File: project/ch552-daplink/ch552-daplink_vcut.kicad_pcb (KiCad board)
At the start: 2 copper layers, 92 x 92 mm, 512 parts, among them J1 USB_C_Receptacle_USB2.0_16P, J10 USB_C_Receptacle_USB2.0_16P, J11 Conn_01x06_Pin, J12 BOOT, J13 USB_C_Receptacle_USB2.0_16P, J14 Conn_01x06_Pin, J15 BOOT, J16 USB_C_Receptacle_USB2.0_16P, J17 Conn_01x06_Pin, J18 BOOT, J19 USB_C_Receptacle_USB2.0_16P, J2 Conn_01x06_Pin, J20 Conn_01x06_Pin, J21 BOOT, J22 USB_C_Receptacle_USB2.0_16P, J23 Conn_01x06_Pin, J24 BOOT, J25 USB_C_Receptacle_USB2.0_16P, J26 Conn_01x06_Pin, J27 BOOT, J28 USB_C_Receptacle_USB2.0_16P, J29 Conn_01x06_Pin, J3 BOOT, J30 BOOT, J31 USB_C_Receptacle_USB2.0_16P, J32 Conn_01x06_Pin, J33 BOOT, J34 USB_C_Receptacle_USB2.0_16P, J35 Conn_01x06_Pin, J36 BOOT, J37 USB_C_Receptacle_USB2.0_16P, J38 Conn_01x06_Pin, J39 BOOT, J4 USB_C_Receptacle_USB2.0_16P, J40 USB_C_Receptacle_USB2.0_16P, J41 Conn_01x06_Pin, J42 BOOT, J43 USB_C_Receptacle_USB2.0_16P, J44 Conn_01x06_Pin, J45 BOOT, J46 USB_C_Receptacle_USB2.0_16P, J47 Conn_01x06_Pin, J48 BOOT, J49 USB_C_Receptacle_USB2.0_16P, J5 Conn_01x06_Pin, J50 Conn_01x06_Pin, J51 BOOT, J52 USB_C_Receptacle_USB2.0_16P, J53 Conn_01x06_Pin, J54 BOOT, J55 USB_C_Receptacle_USB2.0_16P, J56 Conn_01x06_Pin, J57 BOOT, J58 USB_C_Receptacle_USB2.0_16P, J59 Conn_01x06_Pin, J6 BOOT, J60 BOOT, J61 USB_C_Receptacle_USB2.0_16P, J62 Conn_01x06_Pin, J63 BOOT, J64 USB_C_Receptacle_USB2.0_16P, J65 Conn_01x06_Pin, J66 BOOT, J67 USB_C_Receptacle_USB2.0_16P, J68 Conn_01x06_Pin, J69 BOOT, J7 USB_C_Receptacle_USB2.0_16P, J70 USB_C_Receptacle_USB2.0_16P, J71 Conn_01x06_Pin, J72 BOOT, J73 USB_C_Receptacle_USB2.0_16P, J74 Conn_01x06_Pin, J75 BOOT, J76 USB_C_Receptacle_USB2.0_16P, J77 Conn_01x06_Pin, J78 BOOT, J79 USB_C_Receptacle_USB2.0_16P, J8 Conn_01x06_Pin, J80 Conn_01x06_Pin, J81 BOOT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

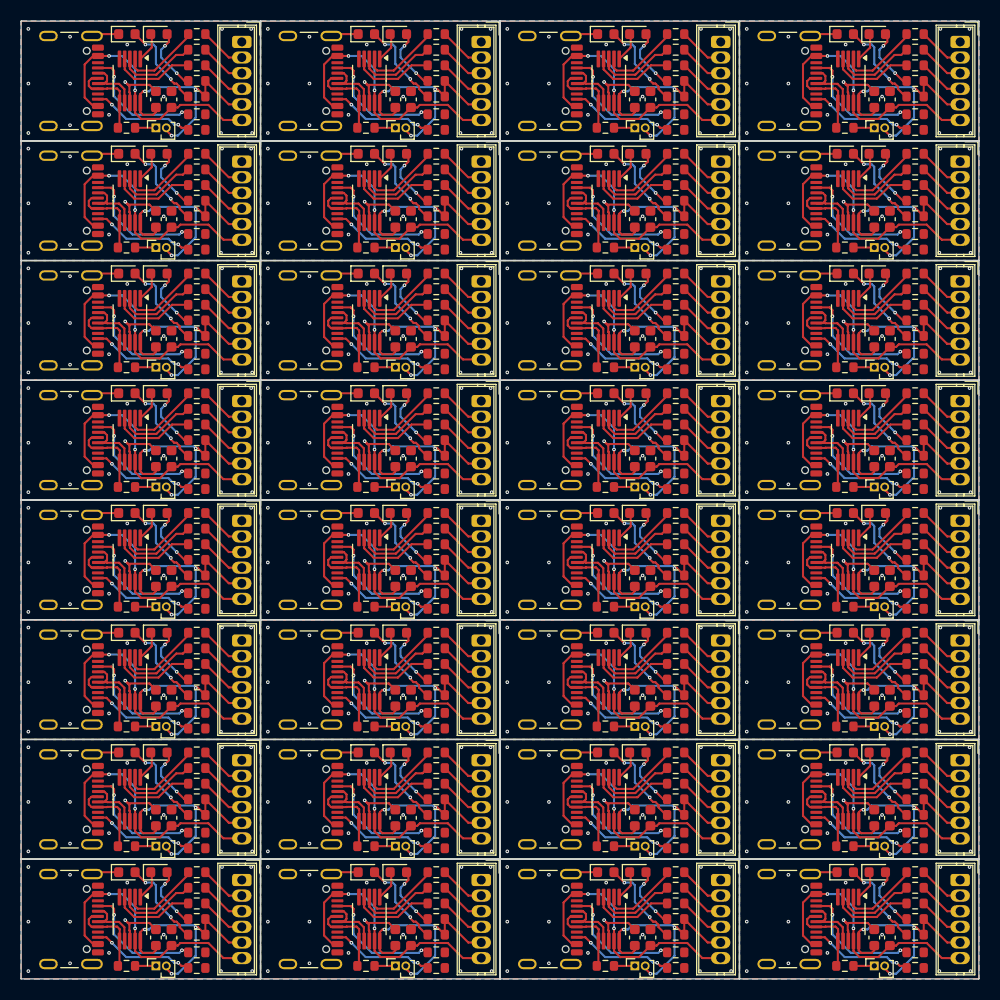
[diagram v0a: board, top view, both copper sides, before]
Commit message: 2025/07/20/17:06
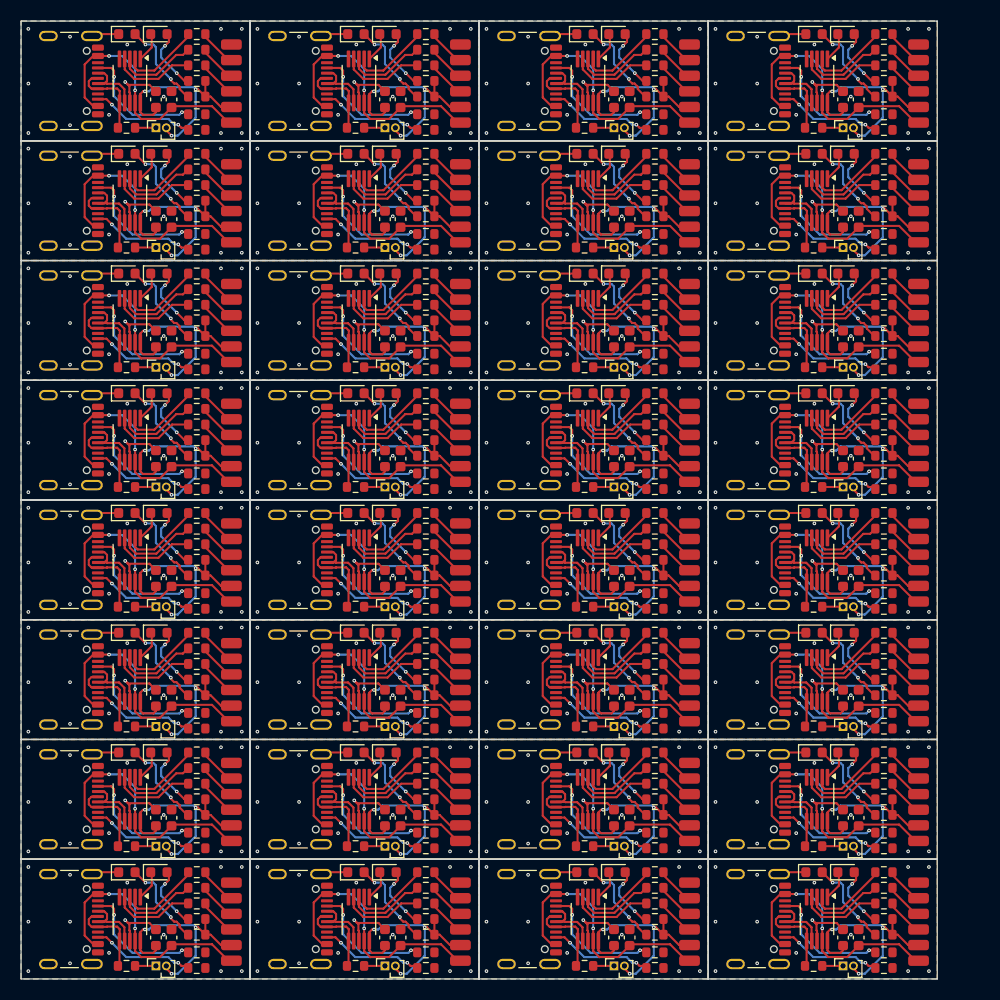
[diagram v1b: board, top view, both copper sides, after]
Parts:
- removed the C1 at (139.4, 175.5)
- removed C10, C11, C12, C13, C14, C15, C16, C17, C18, C19, C20, C21, C22, C23, C24, C25, C26, C27, C28, C29, C3, C30, C31, C32, C33, C34, C35, C36, C37, C38, C39, C4, C40, C41, C42, C43, C44, C45, C46, C47, C48, C49, C5, C50, C51, C52, C53, C54, C55, C56, C57, C58, C59, C6, C60, C61, C62, C63, C64, C7, C8, C9: 0.1uF, Capacitor_SMD:C_0603_1608Metric
- removed the C2 at (140.9, 175.5)
- removed the D1 at (136.7, 169.2)
- removed D10, D12, D14, D16, D18, D20, D22, D24, D26, D28, D30, D32, D34, D36, D38, D4, D40, D42, D44, D46, D48, D50, D52, D54, D56, D58, D6, D60, D62, D64, D8: Green, LED_SMD:LED_0603_1608Metric
- removed D11, D13, D15, D17, D19, D21, D23, D25, D27, D29, D3, D31, D33, D35, D37, D39, D41, D43, D45, D47, D49, D5, D51, D53, D55, D57, D59, D61, D63, D7, D9: Blue, LED_SMD:LED_0603_1608Metric
- removed the D2 at (139.7, 169.2)
- removed the J1 at (130.2, 173.8)
- removed J10, J13, J16, J19, J22, J25, J28, J31, J34, J37, J4, J40, J43, J46, J49, J52, J55, J58, J61, J64, J67, J7, J70, J73, J76, J79, J82, J85, J88, J91, J94: USB_C_Receptacle_USB2.0_16P, Connector_USB:USB_C_Receptacle_GCT_USB4105-xx-A_16P_TopMnt_Horizontal
- removed J11, J14, J17, J2, J20, J23, J26, J29, J32, J35, J38, J41, J44, J47, J5, J50, J53, J56, J59, J62, J65, J68, J71, J74, J77, J8, J80, J83, J86, J89, J92, J95: Conn_01x06_Pin, Connector_Wuerth:Wuerth_WR-WTB_64800611622_1x06_P1.50mm_Vertical
- removed J12, J15, J18, J21, J24, J27, J30, J33, J36, J39, J42, J45, J48, J51, J54, J57, J6, J60, J63, J66, J69, J72, J75, J78, J81, J84, J87, J9, J90, J93, J96: BOOT, Connector_PinSocket_1.00mm:PinSocket_1x02_P1.00mm_Vertical
- removed the J3 at (139.4, 178.2)
- removed the R1 at (143.4, 176.9)
- removed R10, R105, R106, R113, R114, R121, R122, R129, R130, R137, R138, R145, R146, R153, R154, R161, R162, R169, R17, R170, R177, R178, R18, R185, R186, R193, R194, R201, R202, R209, R210, R217, R218, R225, R226, R233, R234, R241, R242, R249, R25, R250, R26, R33, R34, R41, R42, R49, R50, R57, R58, R65, R66, R73, R74, R81, R82, R89, R9, R90, R97, R98: 5.1kΩ, Resistor_SMD:R_0603_1608Metric
- removed R100, R107, R108, R11, R115, R116, R12, R123, R124, R131, R132, R139, R140, R147, R148, R155, R156, R163, R164, R171, R172, R179, R180, R187, R188, R19, R195, R196, R20, R203, R204, R211, R212, R219, R220, R227, R228, R235, R236, R243, R244, R251, R252, R27, R28, R35, R36, R43, R44, R51, R52, R59, R60, R67, R68, R75, R76, R83, R84, R91, R92, R99: 1kΩ, Resistor_SMD:R_0603_1608Metric
- removed R101, R109, R117, R125, R13, R133, R141, R149, R157, R165, R173, R181, R189, R197, R205, R21, R213, R221, R229, R237, R245, R253, R29, R37, R45, R53, R61, R69, R77, R85, R93: 10kΩ, Resistor_SMD:R_0603_1608Metric
- removed R102, R103, R104, R110, R111, R112, R118, R119, R120, R126, R127, R128, R134, R135, R136, R14, R142, R143, R144, R15, R150, R151, R152, R158, R159, R16, R160, R166, R167, R168, R174, R175, R176, R182, R183, R184, R190, R191, R192, R198, R199, R200, R206, R207, R208, R214, R215, R216, R22, R222, R223, R224, R23, R230, R231, R232, R238, R239, R24, R240, R246, R247, R248, R254, R255, R256, R30, R31, R32, R38, R39, R40, R46, R47, R48, R54, R55, R56, R62, R63, R64, R70, R71, R72, R78, R79, R80, R86, R87, R88, R94, R95, R96: 100Ω, Resistor_SMD:R_0603_1608Metric
- removed the R2 at (143.4, 178.4)
- removed the R3 at (143.4, 175.2)
- removed the R4 at (143.4, 173.8)
- removed the R5 at (136.6, 178.2)
- removed the R6 at (143.4, 172.2)
- removed the R7 at (143.4, 170.8)
- removed the R8 at (143.4, 169.2)
- removed the U1 at (136.9, 173.8)
- removed U10, U11, U12, U13, U14, U15, U16, U17, U18, U19, U2, U20, U21, U22, U23, U24, U25, U26, U27, U28, U29, U3, U30, U31, U32, U4, U5, U6, U7, U8, U9: CH552E, Package_SO:MSOP-10_3x3mm_P0.5mm
- added C1: 0.1uF, Capacitor_SMD:C_0603_1608Metric, F.Cu at (92.5, 95.0)
- added C1: 0.1uF, Capacitor_SMD:C_0603_1608Metric, F.Cu at (92.5, 106.5)
- added C1: 0.1uF, Capacitor_SMD:C_0603_1608Metric, F.Cu at (70.5, 164.0)
- added C1: 0.1uF, Capacitor_SMD:C_0603_1608Metric, F.Cu at (70.5, 106.5)
- added C1: 0.1uF, Capacitor_SMD:C_0603_1608Metric, F.Cu at (136.4, 175.5)
- added C1: 0.1uF, Capacitor_SMD:C_0603_1608Metric, F.Cu at (92.5, 164.0)
- added C1: 0.1uF, Capacitor_SMD:C_0603_1608Metric, F.Cu at (70.5, 118.0)
- added C1: 0.1uF, Capacitor_SMD:C_0603_1608Metric, F.Cu at (70.5, 152.5)
- added C1: 0.1uF, Capacitor_SMD:C_0603_1608Metric, F.Cu at (92.5, 118.0)
- added C1: 0.1uF, Capacitor_SMD:C_0603_1608Metric, F.Cu at (114.5, 129.5)
- added C1: 0.1uF, Capacitor_SMD:C_0603_1608Metric, F.Cu at (136.4, 164.0)
- added C1: 0.1uF, Capacitor_SMD:C_0603_1608Metric, F.Cu at (114.5, 152.5)
- added C1: 0.1uF, Capacitor_SMD:C_0603_1608Metric, F.Cu at (70.5, 129.5)
- added C1: 0.1uF, Capacitor_SMD:C_0603_1608Metric, F.Cu at (114.5, 118.0)
- added C1: 0.1uF, Capacitor_SMD:C_0603_1608Metric, F.Cu at (136.4, 95.0)
- added C1: 0.1uF, Capacitor_SMD:C_0603_1608Metric, F.Cu at (70.5, 141.0)
- added C1: 0.1uF, Capacitor_SMD:C_0603_1608Metric, F.Cu at (136.4, 152.5)
- added C1: 0.1uF, Capacitor_SMD:C_0603_1608Metric, F.Cu at (114.5, 95.0)
- added C1: 0.1uF, Capacitor_SMD:C_0603_1608Metric, F.Cu at (92.5, 129.5)
- added C1: 0.1uF, Capacitor_SMD:C_0603_1608Metric, F.Cu at (136.4, 129.5)
- added C1: 0.1uF, Capacitor_SMD:C_0603_1608Metric, F.Cu at (92.5, 141.0)
- added C1: 0.1uF, Capacitor_SMD:C_0603_1608Metric, F.Cu at (70.5, 175.5)
- added C1: 0.1uF, Capacitor_SMD:C_0603_1608Metric, F.Cu at (92.5, 175.5)
- added C1: 0.1uF, Capacitor_SMD:C_0603_1608Metric, F.Cu at (92.5, 152.5)
- added C1: 0.1uF, Capacitor_SMD:C_0603_1608Metric, F.Cu at (136.4, 106.5)
- added C1: 0.1uF, Capacitor_SMD:C_0603_1608Metric, F.Cu at (114.5, 106.5)
- added C1: 0.1uF, Capacitor_SMD:C_0603_1608Metric, F.Cu at (70.5, 95.0)
- added C1: 0.1uF, Capacitor_SMD:C_0603_1608Metric, F.Cu at (136.4, 118.0)
- added C1: 0.1uF, Capacitor_SMD:C_0603_1608Metric, F.Cu at (114.5, 164.0)
- added C1: 0.1uF, Capacitor_SMD:C_0603_1608Metric, F.Cu at (114.5, 141.0)
- added C1: 0.1uF, Capacitor_SMD:C_0603_1608Metric, F.Cu at (114.5, 175.5)
- added C1: 0.1uF, Capacitor_SMD:C_0603_1608Metric, F.Cu at (136.4, 141.0)
- added C2: 0.1uF, Capacitor_SMD:C_0603_1608Metric, F.Cu at (116.0, 152.5)
- added C2: 0.1uF, Capacitor_SMD:C_0603_1608Metric, F.Cu at (94.0, 118.0)
- added C2: 0.1uF, Capacitor_SMD:C_0603_1608Metric, F.Cu at (116.0, 141.0)
- added C2: 0.1uF, Capacitor_SMD:C_0603_1608Metric, F.Cu at (94.0, 106.5)
- added C2: 0.1uF, Capacitor_SMD:C_0603_1608Metric, F.Cu at (137.9, 152.5)
- added C2: 0.1uF, Capacitor_SMD:C_0603_1608Metric, F.Cu at (72.0, 129.5)
- added C2: 0.1uF, Capacitor_SMD:C_0603_1608Metric, F.Cu at (72.0, 95.0)
- added C2: 0.1uF, Capacitor_SMD:C_0603_1608Metric, F.Cu at (137.9, 95.0)
- added C2: 0.1uF, Capacitor_SMD:C_0603_1608Metric, F.Cu at (116.0, 164.0)
- added C2: 0.1uF, Capacitor_SMD:C_0603_1608Metric, F.Cu at (72.0, 175.5)
- added C2: 0.1uF, Capacitor_SMD:C_0603_1608Metric, F.Cu at (116.0, 129.5)
- added C2: 0.1uF, Capacitor_SMD:C_0603_1608Metric, F.Cu at (116.0, 95.0)
- added C2: 0.1uF, Capacitor_SMD:C_0603_1608Metric, F.Cu at (116.0, 106.5)
- added C2: 0.1uF, Capacitor_SMD:C_0603_1608Metric, F.Cu at (94.0, 175.5)
- added C2: 0.1uF, Capacitor_SMD:C_0603_1608Metric, F.Cu at (94.0, 129.5)
- added C2: 0.1uF, Capacitor_SMD:C_0603_1608Metric, F.Cu at (94.0, 95.0)
- added C2: 0.1uF, Capacitor_SMD:C_0603_1608Metric, F.Cu at (72.0, 118.0)
- added C2: 0.1uF, Capacitor_SMD:C_0603_1608Metric, F.Cu at (137.9, 141.0)
- added C2: 0.1uF, Capacitor_SMD:C_0603_1608Metric, F.Cu at (137.9, 106.5)
- added C2: 0.1uF, Capacitor_SMD:C_0603_1608Metric, F.Cu at (116.0, 118.0)
- added C2: 0.1uF, Capacitor_SMD:C_0603_1608Metric, F.Cu at (72.0, 164.0)
- added C2: 0.1uF, Capacitor_SMD:C_0603_1608Metric, F.Cu at (94.0, 164.0)
- added C2: 0.1uF, Capacitor_SMD:C_0603_1608Metric, F.Cu at (137.9, 118.0)
- added C2: 0.1uF, Capacitor_SMD:C_0603_1608Metric, F.Cu at (94.0, 152.5)
- added C2: 0.1uF, Capacitor_SMD:C_0603_1608Metric, F.Cu at (72.0, 141.0)
- added C2: 0.1uF, Capacitor_SMD:C_0603_1608Metric, F.Cu at (137.9, 164.0)
- added C2: 0.1uF, Capacitor_SMD:C_0603_1608Metric, F.Cu at (72.0, 106.5)
- added C2: 0.1uF, Capacitor_SMD:C_0603_1608Metric, F.Cu at (72.0, 152.5)
- added C2: 0.1uF, Capacitor_SMD:C_0603_1608Metric, F.Cu at (116.0, 175.5)
- added C2: 0.1uF, Capacitor_SMD:C_0603_1608Metric, F.Cu at (137.9, 129.5)
- added C2: 0.1uF, Capacitor_SMD:C_0603_1608Metric, F.Cu at (94.0, 141.0)
- added C2: 0.1uF, Capacitor_SMD:C_0603_1608Metric, F.Cu at (137.9, 175.5)
- added D1: Blue, LED_SMD:LED_0603_1608Metric, F.Cu at (133.7, 146.2)
- added D1: Blue, LED_SMD:LED_0603_1608Metric, F.Cu at (133.7, 123.2)
- added D1: Blue, LED_SMD:LED_0603_1608Metric, F.Cu at (89.7, 100.2)
- added D1: Blue, LED_SMD:LED_0603_1608Metric, F.Cu at (133.7, 88.8)
- added D1: Blue, LED_SMD:LED_0603_1608Metric, F.Cu at (67.7, 146.2)
- added D1: Blue, LED_SMD:LED_0603_1608Metric, F.Cu at (133.7, 169.2)
- added D1: Blue, LED_SMD:LED_0603_1608Metric, F.Cu at (133.7, 111.8)
- added D1: Blue, LED_SMD:LED_0603_1608Metric, F.Cu at (89.7, 123.2)
- added D1: Blue, LED_SMD:LED_0603_1608Metric, F.Cu at (133.7, 100.2)
- added D1: Blue, LED_SMD:LED_0603_1608Metric, F.Cu at (67.7, 123.2)
- added D1: Blue, LED_SMD:LED_0603_1608Metric, F.Cu at (111.7, 169.2)
- added D1: Blue, LED_SMD:LED_0603_1608Metric, F.Cu at (67.7, 100.2)
- added D1: Blue, LED_SMD:LED_0603_1608Metric, F.Cu at (67.7, 88.8)
- added D1: Blue, LED_SMD:LED_0603_1608Metric, F.Cu at (89.7, 88.8)
- added D1: Blue, LED_SMD:LED_0603_1608Metric, F.Cu at (89.7, 146.2)
- added D1: Blue, LED_SMD:LED_0603_1608Metric, F.Cu at (111.7, 100.2)
- added D1: Blue, LED_SMD:LED_0603_1608Metric, F.Cu at (111.7, 123.2)
- added D1: Blue, LED_SMD:LED_0603_1608Metric, F.Cu at (111.7, 111.8)
- added D1: Blue, LED_SMD:LED_0603_1608Metric, F.Cu at (111.7, 88.8)
- added D1: Blue, LED_SMD:LED_0603_1608Metric, F.Cu at (89.7, 134.8)
- added D1: Blue, LED_SMD:LED_0603_1608Metric, F.Cu at (133.7, 134.8)
- added D1: Blue, LED_SMD:LED_0603_1608Metric, F.Cu at (67.7, 111.8)
- added D1: Blue, LED_SMD:LED_0603_1608Metric, F.Cu at (89.7, 111.8)
- added D1: Blue, LED_SMD:LED_0603_1608Metric, F.Cu at (89.7, 169.2)
- added D1: Blue, LED_SMD:LED_0603_1608Metric, F.Cu at (111.7, 157.8)
- added D1: Blue, LED_SMD:LED_0603_1608Metric, F.Cu at (67.7, 134.8)
- added D1: Blue, LED_SMD:LED_0603_1608Metric, F.Cu at (133.7, 157.8)
- added D1: Blue, LED_SMD:LED_0603_1608Metric, F.Cu at (67.7, 169.2)
- added D1: Blue, LED_SMD:LED_0603_1608Metric, F.Cu at (89.7, 157.8)
- added D1: Blue, LED_SMD:LED_0603_1608Metric, F.Cu at (67.7, 157.8)
- added D1: Blue, LED_SMD:LED_0603_1608Metric, F.Cu at (111.7, 134.8)
- added D1: Blue, LED_SMD:LED_0603_1608Metric, F.Cu at (111.7, 146.2)
- added D2: Green, LED_SMD:LED_0603_1608Metric, F.Cu at (92.7, 100.2)
- added D2: Green, LED_SMD:LED_0603_1608Metric, F.Cu at (136.7, 134.8)
- added D2: Green, LED_SMD:LED_0603_1608Metric, F.Cu at (136.7, 157.8)
- added D2: Green, LED_SMD:LED_0603_1608Metric, F.Cu at (92.7, 146.2)
- added D2: Green, LED_SMD:LED_0603_1608Metric, F.Cu at (114.7, 111.8)
- added D2: Green, LED_SMD:LED_0603_1608Metric, F.Cu at (70.7, 88.8)
- added D2: Green, LED_SMD:LED_0603_1608Metric, F.Cu at (70.7, 157.8)
- added D2: Green, LED_SMD:LED_0603_1608Metric, F.Cu at (114.7, 134.8)
- added D2: Green, LED_SMD:LED_0603_1608Metric, F.Cu at (136.7, 88.8)
- added D2: Green, LED_SMD:LED_0603_1608Metric, F.Cu at (92.7, 157.8)
- added D2: Green, LED_SMD:LED_0603_1608Metric, F.Cu at (70.7, 123.2)
- added D2: Green, LED_SMD:LED_0603_1608Metric, F.Cu at (70.7, 111.8)
- added D2: Green, LED_SMD:LED_0603_1608Metric, F.Cu at (114.7, 88.8)
- added D2: Green, LED_SMD:LED_0603_1608Metric, F.Cu at (92.7, 134.8)
- added D2: Green, LED_SMD:LED_0603_1608Metric, F.Cu at (70.7, 169.2)
- added D2: Green, LED_SMD:LED_0603_1608Metric, F.Cu at (136.7, 146.2)
- added D2: Green, LED_SMD:LED_0603_1608Metric, F.Cu at (92.7, 123.2)
- added D2: Green, LED_SMD:LED_0603_1608Metric, F.Cu at (136.7, 169.2)
- added D2: Green, LED_SMD:LED_0603_1608Metric, F.Cu at (136.7, 123.2)
- added D2: Green, LED_SMD:LED_0603_1608Metric, F.Cu at (114.7, 123.2)
- added D2: Green, LED_SMD:LED_0603_1608Metric, F.Cu at (70.7, 134.8)
- added D2: Green, LED_SMD:LED_0603_1608Metric, F.Cu at (114.7, 169.2)
- added D2: Green, LED_SMD:LED_0603_1608Metric, F.Cu at (114.7, 146.2)
- added D2: Green, LED_SMD:LED_0603_1608Metric, F.Cu at (92.7, 88.8)
- added D2: Green, LED_SMD:LED_0603_1608Metric, F.Cu at (136.7, 100.2)
- added D2: Green, LED_SMD:LED_0603_1608Metric, F.Cu at (70.7, 100.2)
- added D2: Green, LED_SMD:LED_0603_1608Metric, F.Cu at (70.7, 146.2)
- added D2: Green, LED_SMD:LED_0603_1608Metric, F.Cu at (92.7, 169.2)
- added D2: Green, LED_SMD:LED_0603_1608Metric, F.Cu at (92.7, 111.8)
- added D2: Green, LED_SMD:LED_0603_1608Metric, F.Cu at (114.7, 157.8)
- added D2: Green, LED_SMD:LED_0603_1608Metric, F.Cu at (136.7, 111.8)
- added D2: Green, LED_SMD:LED_0603_1608Metric, F.Cu at (114.7, 100.2)
- added J1: USB_C_Receptacle_USB2.0_16P, Connector_USB:USB_C_Receptacle_GCT_USB4105-xx-A_16P_TopMnt_Horizontal, F.Cu at (61.2, 104.8)
- added J1: USB_C_Receptacle_USB2.0_16P, Connector_USB:USB_C_Receptacle_GCT_USB4105-xx-A_16P_TopMnt_Horizontal, F.Cu at (83.2, 93.2)
- added J1: USB_C_Receptacle_USB2.0_16P, Connector_USB:USB_C_Receptacle_GCT_USB4105-xx-A_16P_TopMnt_Horizontal, F.Cu at (127.2, 93.2)
- added J1: USB_C_Receptacle_USB2.0_16P, Connector_USB:USB_C_Receptacle_GCT_USB4105-xx-A_16P_TopMnt_Horizontal, F.Cu at (61.2, 162.2)
- added J1: USB_C_Receptacle_USB2.0_16P, Connector_USB:USB_C_Receptacle_GCT_USB4105-xx-A_16P_TopMnt_Horizontal, F.Cu at (105.2, 150.8)
- added J1: USB_C_Receptacle_USB2.0_16P, Connector_USB:USB_C_Receptacle_GCT_USB4105-xx-A_16P_TopMnt_Horizontal, F.Cu at (127.2, 150.8)
- added J1: USB_C_Receptacle_USB2.0_16P, Connector_USB:USB_C_Receptacle_GCT_USB4105-xx-A_16P_TopMnt_Horizontal, F.Cu at (105.2, 104.8)
- added J1: USB_C_Receptacle_USB2.0_16P, Connector_USB:USB_C_Receptacle_GCT_USB4105-xx-A_16P_TopMnt_Horizontal, F.Cu at (127.2, 139.2)
- added J1: USB_C_Receptacle_USB2.0_16P, Connector_USB:USB_C_Receptacle_GCT_USB4105-xx-A_16P_TopMnt_Horizontal, F.Cu at (127.2, 173.8)
- added J1: USB_C_Receptacle_USB2.0_16P, Connector_USB:USB_C_Receptacle_GCT_USB4105-xx-A_16P_TopMnt_Horizontal, F.Cu at (61.2, 127.8)
- added J1: USB_C_Receptacle_USB2.0_16P, Connector_USB:USB_C_Receptacle_GCT_USB4105-xx-A_16P_TopMnt_Horizontal, F.Cu at (61.2, 116.2)
- added J1: USB_C_Receptacle_USB2.0_16P, Connector_USB:USB_C_Receptacle_GCT_USB4105-xx-A_16P_TopMnt_Horizontal, F.Cu at (61.2, 139.2)
- added J1: USB_C_Receptacle_USB2.0_16P, Connector_USB:USB_C_Receptacle_GCT_USB4105-xx-A_16P_TopMnt_Horizontal, F.Cu at (105.2, 127.8)
- added J1: USB_C_Receptacle_USB2.0_16P, Connector_USB:USB_C_Receptacle_GCT_USB4105-xx-A_16P_TopMnt_Horizontal, F.Cu at (105.2, 173.8)
- added J1: USB_C_Receptacle_USB2.0_16P, Connector_USB:USB_C_Receptacle_GCT_USB4105-xx-A_16P_TopMnt_Horizontal, F.Cu at (105.2, 139.2)
- added J1: USB_C_Receptacle_USB2.0_16P, Connector_USB:USB_C_Receptacle_GCT_USB4105-xx-A_16P_TopMnt_Horizontal, F.Cu at (83.2, 127.8)
- added J1: USB_C_Receptacle_USB2.0_16P, Connector_USB:USB_C_Receptacle_GCT_USB4105-xx-A_16P_TopMnt_Horizontal, F.Cu at (105.2, 116.2)
- added J1: USB_C_Receptacle_USB2.0_16P, Connector_USB:USB_C_Receptacle_GCT_USB4105-xx-A_16P_TopMnt_Horizontal, F.Cu at (83.2, 116.2)
- added J1: USB_C_Receptacle_USB2.0_16P, Connector_USB:USB_C_Receptacle_GCT_USB4105-xx-A_16P_TopMnt_Horizontal, F.Cu at (61.2, 93.2)
- added J1: USB_C_Receptacle_USB2.0_16P, Connector_USB:USB_C_Receptacle_GCT_USB4105-xx-A_16P_TopMnt_Horizontal, F.Cu at (83.2, 139.2)
- added J1: USB_C_Receptacle_USB2.0_16P, Connector_USB:USB_C_Receptacle_GCT_USB4105-xx-A_16P_TopMnt_Horizontal, F.Cu at (83.2, 162.2)
- added J1: USB_C_Receptacle_USB2.0_16P, Connector_USB:USB_C_Receptacle_GCT_USB4105-xx-A_16P_TopMnt_Horizontal, F.Cu at (83.2, 150.8)
- added J1: USB_C_Receptacle_USB2.0_16P, Connector_USB:USB_C_Receptacle_GCT_USB4105-xx-A_16P_TopMnt_Horizontal, F.Cu at (127.2, 116.2)
- added J1: USB_C_Receptacle_USB2.0_16P, Connector_USB:USB_C_Receptacle_GCT_USB4105-xx-A_16P_TopMnt_Horizontal, F.Cu at (127.2, 104.8)
- added J1: USB_C_Receptacle_USB2.0_16P, Connector_USB:USB_C_Receptacle_GCT_USB4105-xx-A_16P_TopMnt_Horizontal, F.Cu at (105.2, 162.2)
- added J1: USB_C_Receptacle_USB2.0_16P, Connector_USB:USB_C_Receptacle_GCT_USB4105-xx-A_16P_TopMnt_Horizontal, F.Cu at (105.2, 93.2)
- added J1: USB_C_Receptacle_USB2.0_16P, Connector_USB:USB_C_Receptacle_GCT_USB4105-xx-A_16P_TopMnt_Horizontal, F.Cu at (127.2, 127.8)
- added J1: USB_C_Receptacle_USB2.0_16P, Connector_USB:USB_C_Receptacle_GCT_USB4105-xx-A_16P_TopMnt_Horizontal, F.Cu at (83.2, 173.8)
- added J1: USB_C_Receptacle_USB2.0_16P, Connector_USB:USB_C_Receptacle_GCT_USB4105-xx-A_16P_TopMnt_Horizontal, F.Cu at (61.2, 173.8)
- added J1: USB_C_Receptacle_USB2.0_16P, Connector_USB:USB_C_Receptacle_GCT_USB4105-xx-A_16P_TopMnt_Horizontal, F.Cu at (127.2, 162.2)
- added J1: USB_C_Receptacle_USB2.0_16P, Connector_USB:USB_C_Receptacle_GCT_USB4105-xx-A_16P_TopMnt_Horizontal, F.Cu at (61.2, 150.8)
- added J1: USB_C_Receptacle_USB2.0_16P, Connector_USB:USB_C_Receptacle_GCT_USB4105-xx-A_16P_TopMnt_Horizontal, F.Cu at (83.2, 104.8)
- added J3: BOOT, Connector_PinSocket_1.00mm:PinSocket_1x02_P1.00mm_Vertical, F.Cu at (70.5, 132.2)
- added J3: BOOT, Connector_PinSocket_1.00mm:PinSocket_1x02_P1.00mm_Vertical, F.Cu at (92.5, 155.2)
- added J3: BOOT, Connector_PinSocket_1.00mm:PinSocket_1x02_P1.00mm_Vertical, F.Cu at (70.5, 143.8)
- added J3: BOOT, Connector_PinSocket_1.00mm:PinSocket_1x02_P1.00mm_Vertical, F.Cu at (70.5, 97.8)
- added J3: BOOT, Connector_PinSocket_1.00mm:PinSocket_1x02_P1.00mm_Vertical, F.Cu at (114.5, 178.2)
- added J3: BOOT, Connector_PinSocket_1.00mm:PinSocket_1x02_P1.00mm_Vertical, F.Cu at (70.5, 120.8)
- added J3: BOOT, Connector_PinSocket_1.00mm:PinSocket_1x02_P1.00mm_Vertical, F.Cu at (136.4, 178.2)
- added J3: BOOT, Connector_PinSocket_1.00mm:PinSocket_1x02_P1.00mm_Vertical, F.Cu at (114.5, 97.8)
- added J3: BOOT, Connector_PinSocket_1.00mm:PinSocket_1x02_P1.00mm_Vertical, F.Cu at (92.5, 109.2)
- added J3: BOOT, Connector_PinSocket_1.00mm:PinSocket_1x02_P1.00mm_Vertical, F.Cu at (70.5, 166.8)
- added J3: BOOT, Connector_PinSocket_1.00mm:PinSocket_1x02_P1.00mm_Vertical, F.Cu at (70.5, 109.2)
- added J3: BOOT, Connector_PinSocket_1.00mm:PinSocket_1x02_P1.00mm_Vertical, F.Cu at (136.4, 166.8)
- added J3: BOOT, Connector_PinSocket_1.00mm:PinSocket_1x02_P1.00mm_Vertical, F.Cu at (70.5, 155.2)
- added J3: BOOT, Connector_PinSocket_1.00mm:PinSocket_1x02_P1.00mm_Vertical, F.Cu at (114.5, 143.8)
- added J3: BOOT, Connector_PinSocket_1.00mm:PinSocket_1x02_P1.00mm_Vertical, F.Cu at (136.4, 132.2)
- added J3: BOOT, Connector_PinSocket_1.00mm:PinSocket_1x02_P1.00mm_Vertical, F.Cu at (136.4, 97.8)
- added J3: BOOT, Connector_PinSocket_1.00mm:PinSocket_1x02_P1.00mm_Vertical, F.Cu at (114.5, 120.8)
- added J3: BOOT, Connector_PinSocket_1.00mm:PinSocket_1x02_P1.00mm_Vertical, F.Cu at (92.5, 97.8)
- added J3: BOOT, Connector_PinSocket_1.00mm:PinSocket_1x02_P1.00mm_Vertical, F.Cu at (92.5, 178.2)
- added J3: BOOT, Connector_PinSocket_1.00mm:PinSocket_1x02_P1.00mm_Vertical, F.Cu at (70.5, 178.2)
- added J3: BOOT, Connector_PinSocket_1.00mm:PinSocket_1x02_P1.00mm_Vertical, F.Cu at (92.5, 120.8)
- added J3: BOOT, Connector_PinSocket_1.00mm:PinSocket_1x02_P1.00mm_Vertical, F.Cu at (92.5, 132.2)
- added J3: BOOT, Connector_PinSocket_1.00mm:PinSocket_1x02_P1.00mm_Vertical, F.Cu at (136.4, 120.8)
- added J3: BOOT, Connector_PinSocket_1.00mm:PinSocket_1x02_P1.00mm_Vertical, F.Cu at (92.5, 143.8)
- added J3: BOOT, Connector_PinSocket_1.00mm:PinSocket_1x02_P1.00mm_Vertical, F.Cu at (136.4, 155.2)
- added J3: BOOT, Connector_PinSocket_1.00mm:PinSocket_1x02_P1.00mm_Vertical, F.Cu at (114.5, 132.2)
- added J3: BOOT, Connector_PinSocket_1.00mm:PinSocket_1x02_P1.00mm_Vertical, F.Cu at (136.4, 143.8)
- added J3: BOOT, Connector_PinSocket_1.00mm:PinSocket_1x02_P1.00mm_Vertical, F.Cu at (92.5, 166.8)
- added J3: BOOT, Connector_PinSocket_1.00mm:PinSocket_1x02_P1.00mm_Vertical, F.Cu at (114.5, 166.8)
- added J3: BOOT, Connector_PinSocket_1.00mm:PinSocket_1x02_P1.00mm_Vertical, F.Cu at (114.5, 109.2)
- added J3: BOOT, Connector_PinSocket_1.00mm:PinSocket_1x02_P1.00mm_Vertical, F.Cu at (114.5, 155.2)
- added J3: BOOT, Connector_PinSocket_1.00mm:PinSocket_1x02_P1.00mm_Vertical, F.Cu at (136.4, 109.2)
- added R1: 5.1kΩ, Resistor_SMD:R_0603_1608Metric, F.Cu at (140.4, 108.0)
- added R1: 5.1kΩ, Resistor_SMD:R_0603_1608Metric, F.Cu at (74.4, 153.9)
- added R1: 5.1kΩ, Resistor_SMD:R_0603_1608Metric, F.Cu at (96.4, 119.5)
- added R1: 5.1kΩ, Resistor_SMD:R_0603_1608Metric, F.Cu at (140.4, 130.9)
- added R1: 5.1kΩ, Resistor_SMD:R_0603_1608Metric, F.Cu at (140.4, 96.5)
- added R1: 5.1kΩ, Resistor_SMD:R_0603_1608Metric, F.Cu at (74.4, 96.5)
- added R1: 5.1kΩ, Resistor_SMD:R_0603_1608Metric, F.Cu at (118.4, 176.9)
- added R1: 5.1kΩ, Resistor_SMD:R_0603_1608Metric, F.Cu at (96.4, 153.9)
- added R1: 5.1kΩ, Resistor_SMD:R_0603_1608Metric, F.Cu at (140.4, 142.4)
- added R1: 5.1kΩ, Resistor_SMD:R_0603_1608Metric, F.Cu at (74.4, 176.9)
- added R1: 5.1kΩ, Resistor_SMD:R_0603_1608Metric, F.Cu at (118.4, 142.4)
- added R1: 5.1kΩ, Resistor_SMD:R_0603_1608Metric, F.Cu at (118.4, 108.0)
- added R1: 5.1kΩ, Resistor_SMD:R_0603_1608Metric, F.Cu at (74.4, 119.5)
- added R1: 5.1kΩ, Resistor_SMD:R_0603_1608Metric, F.Cu at (118.4, 153.9)
- added R1: 5.1kΩ, Resistor_SMD:R_0603_1608Metric, F.Cu at (74.4, 165.4)
- added R1: 5.1kΩ, Resistor_SMD:R_0603_1608Metric, F.Cu at (96.4, 108.0)
- added R1: 5.1kΩ, Resistor_SMD:R_0603_1608Metric, F.Cu at (96.4, 176.9)
- added R1: 5.1kΩ, Resistor_SMD:R_0603_1608Metric, F.Cu at (96.4, 142.4)
- added R1: 5.1kΩ, Resistor_SMD:R_0603_1608Metric, F.Cu at (118.4, 119.5)
- added R1: 5.1kΩ, Resistor_SMD:R_0603_1608Metric, F.Cu at (140.4, 165.4)
- added R1: 5.1kΩ, Resistor_SMD:R_0603_1608Metric, F.Cu at (74.4, 108.0)
- added R1: 5.1kΩ, Resistor_SMD:R_0603_1608Metric, F.Cu at (74.4, 130.9)
- added R1: 5.1kΩ, Resistor_SMD:R_0603_1608Metric, F.Cu at (140.4, 176.9)
- added R1: 5.1kΩ, Resistor_SMD:R_0603_1608Metric, F.Cu at (96.4, 96.5)
- added R1: 5.1kΩ, Resistor_SMD:R_0603_1608Metric, F.Cu at (118.4, 165.4)
- added R1: 5.1kΩ, Resistor_SMD:R_0603_1608Metric, F.Cu at (118.4, 96.5)
- added R1: 5.1kΩ, Resistor_SMD:R_0603_1608Metric, F.Cu at (96.4, 165.4)
- added R1: 5.1kΩ, Resistor_SMD:R_0603_1608Metric, F.Cu at (118.4, 130.9)
- added R1: 5.1kΩ, Resistor_SMD:R_0603_1608Metric, F.Cu at (140.4, 119.5)
- added R1: 5.1kΩ, Resistor_SMD:R_0603_1608Metric, F.Cu at (74.4, 142.4)
- added R1: 5.1kΩ, Resistor_SMD:R_0603_1608Metric, F.Cu at (96.4, 130.9)
- added R1: 5.1kΩ, Resistor_SMD:R_0603_1608Metric, F.Cu at (140.4, 153.9)
- added R2: 5.1kΩ, Resistor_SMD:R_0603_1608Metric, F.Cu at (118.4, 109.5)
- added R2: 5.1kΩ, Resistor_SMD:R_0603_1608Metric, F.Cu at (74.4, 109.5)
- added R2: 5.1kΩ, Resistor_SMD:R_0603_1608Metric, F.Cu at (96.4, 178.4)
- added R2: 5.1kΩ, Resistor_SMD:R_0603_1608Metric, F.Cu at (96.4, 121.0)
- added R2: 5.1kΩ, Resistor_SMD:R_0603_1608Metric, F.Cu at (74.4, 155.4)
- added R2: 5.1kΩ, Resistor_SMD:R_0603_1608Metric, F.Cu at (96.4, 109.5)
- added R2: 5.1kΩ, Resistor_SMD:R_0603_1608Metric, F.Cu at (118.4, 121.0)
- added R2: 5.1kΩ, Resistor_SMD:R_0603_1608Metric, F.Cu at (96.4, 166.9)
- added R2: 5.1kΩ, Resistor_SMD:R_0603_1608Metric, F.Cu at (140.4, 132.4)
- added R2: 5.1kΩ, Resistor_SMD:R_0603_1608Metric, F.Cu at (140.4, 98.0)
- added R2: 5.1kΩ, Resistor_SMD:R_0603_1608Metric, F.Cu at (140.4, 166.9)
- added R2: 5.1kΩ, Resistor_SMD:R_0603_1608Metric, F.Cu at (118.4, 143.9)
- added R2: 5.1kΩ, Resistor_SMD:R_0603_1608Metric, F.Cu at (118.4, 155.4)
- added R2: 5.1kΩ, Resistor_SMD:R_0603_1608Metric, F.Cu at (96.4, 132.4)
- added R2: 5.1kΩ, Resistor_SMD:R_0603_1608Metric, F.Cu at (96.4, 98.0)
- added R2: 5.1kΩ, Resistor_SMD:R_0603_1608Metric, F.Cu at (140.4, 121.0)
- added R2: 5.1kΩ, Resistor_SMD:R_0603_1608Metric, F.Cu at (118.4, 98.0)
- added R2: 5.1kΩ, Resistor_SMD:R_0603_1608Metric, F.Cu at (74.4, 98.0)
- added R2: 5.1kΩ, Resistor_SMD:R_0603_1608Metric, F.Cu at (96.4, 155.4)
- added R2: 5.1kΩ, Resistor_SMD:R_0603_1608Metric, F.Cu at (140.4, 178.4)
- added R2: 5.1kΩ, Resistor_SMD:R_0603_1608Metric, F.Cu at (74.4, 143.9)
- added R2: 5.1kΩ, Resistor_SMD:R_0603_1608Metric, F.Cu at (74.4, 121.0)
- added R2: 5.1kΩ, Resistor_SMD:R_0603_1608Metric, F.Cu at (118.4, 132.4)
- added R2: 5.1kΩ, Resistor_SMD:R_0603_1608Metric, F.Cu at (140.4, 155.4)
- added R2: 5.1kΩ, Resistor_SMD:R_0603_1608Metric, F.Cu at (74.4, 166.9)
- added R2: 5.1kΩ, Resistor_SMD:R_0603_1608Metric, F.Cu at (140.4, 109.5)
- added R2: 5.1kΩ, Resistor_SMD:R_0603_1608Metric, F.Cu at (74.4, 178.4)
- added R2: 5.1kΩ, Resistor_SMD:R_0603_1608Metric, F.Cu at (118.4, 178.4)
- added R2: 5.1kΩ, Resistor_SMD:R_0603_1608Metric, F.Cu at (118.4, 166.9)
- added R2: 5.1kΩ, Resistor_SMD:R_0603_1608Metric, F.Cu at (96.4, 143.9)
- added R2: 5.1kΩ, Resistor_SMD:R_0603_1608Metric, F.Cu at (140.4, 143.9)
- added R2: 5.1kΩ, Resistor_SMD:R_0603_1608Metric, F.Cu at (74.4, 132.4)
- added R3: 1kΩ, Resistor_SMD:R_0603_1608Metric, F.Cu at (96.4, 152.2)
- added R3: 1kΩ, Resistor_SMD:R_0603_1608Metric, F.Cu at (140.4, 140.8)
- added R3: 1kΩ, Resistor_SMD:R_0603_1608Metric, F.Cu at (74.4, 106.2)
- added R3: 1kΩ, Resistor_SMD:R_0603_1608Metric, F.Cu at (74.4, 129.2)
- added R3: 1kΩ, Resistor_SMD:R_0603_1608Metric, F.Cu at (118.4, 140.8)
- added R3: 1kΩ, Resistor_SMD:R_0603_1608Metric, F.Cu at (118.4, 117.8)
- added R3: 1kΩ, Resistor_SMD:R_0603_1608Metric, F.Cu at (96.4, 94.8)
- added R3: 1kΩ, Resistor_SMD:R_0603_1608Metric, F.Cu at (140.4, 163.8)
- added R3: 1kΩ, Resistor_SMD:R_0603_1608Metric, F.Cu at (140.4, 152.2)
- added R3: 1kΩ, Resistor_SMD:R_0603_1608Metric, F.Cu at (118.4, 163.8)
- added R3: 1kΩ, Resistor_SMD:R_0603_1608Metric, F.Cu at (96.4, 117.8)
- added R3: 1kΩ, Resistor_SMD:R_0603_1608Metric, F.Cu at (96.4, 129.2)
- added R3: 1kΩ, Resistor_SMD:R_0603_1608Metric, F.Cu at (140.4, 94.8)
- added R3: 1kΩ, Resistor_SMD:R_0603_1608Metric, F.Cu at (74.4, 163.8)
- added R3: 1kΩ, Resistor_SMD:R_0603_1608Metric, F.Cu at (96.4, 175.2)
- added R3: 1kΩ, Resistor_SMD:R_0603_1608Metric, F.Cu at (118.4, 129.2)
- added R3: 1kΩ, Resistor_SMD:R_0603_1608Metric, F.Cu at (74.4, 152.2)
- added R3: 1kΩ, Resistor_SMD:R_0603_1608Metric, F.Cu at (96.4, 140.8)
- added R3: 1kΩ, Resistor_SMD:R_0603_1608Metric, F.Cu at (74.4, 140.8)
- added R3: 1kΩ, Resistor_SMD:R_0603_1608Metric, F.Cu at (118.4, 152.2)
- added R3: 1kΩ, Resistor_SMD:R_0603_1608Metric, F.Cu at (74.4, 117.8)
- added R3: 1kΩ, Resistor_SMD:R_0603_1608Metric, F.Cu at (118.4, 175.2)
- added R3: 1kΩ, Resistor_SMD:R_0603_1608Metric, F.Cu at (74.4, 175.2)
- added R3: 1kΩ, Resistor_SMD:R_0603_1608Metric, F.Cu at (140.4, 129.2)
- added R3: 1kΩ, Resistor_SMD:R_0603_1608Metric, F.Cu at (118.4, 94.8)
- added R3: 1kΩ, Resistor_SMD:R_0603_1608Metric, F.Cu at (74.4, 94.8)
- added R3: 1kΩ, Resistor_SMD:R_0603_1608Metric, F.Cu at (118.4, 106.2)
- added R3: 1kΩ, Resistor_SMD:R_0603_1608Metric, F.Cu at (96.4, 106.2)
- added R3: 1kΩ, Resistor_SMD:R_0603_1608Metric, F.Cu at (140.4, 106.2)
- added R3: 1kΩ, Resistor_SMD:R_0603_1608Metric, F.Cu at (140.4, 175.2)
- added R3: 1kΩ, Resistor_SMD:R_0603_1608Metric, F.Cu at (96.4, 163.8)
- added R3: 1kΩ, Resistor_SMD:R_0603_1608Metric, F.Cu at (140.4, 117.8)
- added R4: 1kΩ, Resistor_SMD:R_0603_1608Metric, F.Cu at (118.4, 127.8)
- added R4: 1kΩ, Resistor_SMD:R_0603_1608Metric, F.Cu at (118.4, 150.8)
- added R4: 1kΩ, Resistor_SMD:R_0603_1608Metric, F.Cu at (96.4, 150.8)
- added R4: 1kΩ, Resistor_SMD:R_0603_1608Metric, F.Cu at (74.4, 127.8)
- added R4: 1kΩ, Resistor_SMD:R_0603_1608Metric, F.Cu at (96.4, 127.8)
- added R4: 1kΩ, Resistor_SMD:R_0603_1608Metric, F.Cu at (74.4, 116.2)
- added R4: 1kΩ, Resistor_SMD:R_0603_1608Metric, F.Cu at (140.4, 116.2)
- added R4: 1kΩ, Resistor_SMD:R_0603_1608Metric, F.Cu at (74.4, 104.8)
- added R4: 1kΩ, Resistor_SMD:R_0603_1608Metric, F.Cu at (118.4, 173.8)
- added R4: 1kΩ, Resistor_SMD:R_0603_1608Metric, F.Cu at (118.4, 116.2)
- added R4: 1kΩ, Resistor_SMD:R_0603_1608Metric, F.Cu at (96.4, 162.2)
- added R4: 1kΩ, Resistor_SMD:R_0603_1608Metric, F.Cu at (96.4, 173.8)
- added R4: 1kΩ, Resistor_SMD:R_0603_1608Metric, F.Cu at (140.4, 150.8)
- added R4: 1kΩ, Resistor_SMD:R_0603_1608Metric, F.Cu at (74.4, 173.8)
- added R4: 1kΩ, Resistor_SMD:R_0603_1608Metric, F.Cu at (96.4, 104.8)
- added R4: 1kΩ, Resistor_SMD:R_0603_1608Metric, F.Cu at (96.4, 139.2)
- added R4: 1kΩ, Resistor_SMD:R_0603_1608Metric, F.Cu at (118.4, 162.2)
- added R4: 1kΩ, Resistor_SMD:R_0603_1608Metric, F.Cu at (140.4, 104.8)
- added R4: 1kΩ, Resistor_SMD:R_0603_1608Metric, F.Cu at (118.4, 93.2)
- added R4: 1kΩ, Resistor_SMD:R_0603_1608Metric, F.Cu at (118.4, 104.8)
- added R4: 1kΩ, Resistor_SMD:R_0603_1608Metric, F.Cu at (74.4, 162.2)
- added R4: 1kΩ, Resistor_SMD:R_0603_1608Metric, F.Cu at (140.4, 162.2)
- added R4: 1kΩ, Resistor_SMD:R_0603_1608Metric, F.Cu at (74.4, 139.2)
- added R4: 1kΩ, Resistor_SMD:R_0603_1608Metric, F.Cu at (140.4, 139.2)
- added R4: 1kΩ, Resistor_SMD:R_0603_1608Metric, F.Cu at (74.4, 150.8)
- added R4: 1kΩ, Resistor_SMD:R_0603_1608Metric, F.Cu at (118.4, 139.2)
- added R4: 1kΩ, Resistor_SMD:R_0603_1608Metric, F.Cu at (96.4, 116.2)
- added R4: 1kΩ, Resistor_SMD:R_0603_1608Metric, F.Cu at (140.4, 173.8)
- added R4: 1kΩ, Resistor_SMD:R_0603_1608Metric, F.Cu at (140.4, 127.8)
- added R4: 1kΩ, Resistor_SMD:R_0603_1608Metric, F.Cu at (74.4, 93.2)
- added R4: 1kΩ, Resistor_SMD:R_0603_1608Metric, F.Cu at (96.4, 93.2)
- added R4: 1kΩ, Resistor_SMD:R_0603_1608Metric, F.Cu at (140.4, 93.2)
- added R5: 10kΩ, Resistor_SMD:R_0603_1608Metric, F.Cu at (67.6, 143.8)
- added R5: 10kΩ, Resistor_SMD:R_0603_1608Metric, F.Cu at (67.6, 178.2)
- added R5: 10kΩ, Resistor_SMD:R_0603_1608Metric, F.Cu at (89.6, 155.2)
- added R5: 10kΩ, Resistor_SMD:R_0603_1608Metric, F.Cu at (89.6, 109.2)
- added R5: 10kΩ, Resistor_SMD:R_0603_1608Metric, F.Cu at (111.6, 155.2)
- added R5: 10kΩ, Resistor_SMD:R_0603_1608Metric, F.Cu at (67.6, 120.8)
- added R5: 10kΩ, Resistor_SMD:R_0603_1608Metric, F.Cu at (133.6, 132.2)
- added R5: 10kΩ, Resistor_SMD:R_0603_1608Metric, F.Cu at (133.6, 166.8)
- added R5: 10kΩ, Resistor_SMD:R_0603_1608Metric, F.Cu at (111.6, 97.8)
- added R5: 10kΩ, Resistor_SMD:R_0603_1608Metric, F.Cu at (133.6, 155.2)
- added R5: 10kΩ, Resistor_SMD:R_0603_1608Metric, F.Cu at (67.6, 109.2)
- added R5: 10kΩ, Resistor_SMD:R_0603_1608Metric, F.Cu at (111.6, 120.8)
- added R5: 10kΩ, Resistor_SMD:R_0603_1608Metric, F.Cu at (133.6, 109.2)
- added R5: 10kΩ, Resistor_SMD:R_0603_1608Metric, F.Cu at (89.6, 97.8)
- added R5: 10kΩ, Resistor_SMD:R_0603_1608Metric, F.Cu at (89.6, 120.8)
- added R5: 10kΩ, Resistor_SMD:R_0603_1608Metric, F.Cu at (89.6, 143.8)
- added R5: 10kΩ, Resistor_SMD:R_0603_1608Metric, F.Cu at (67.6, 155.2)
- added R5: 10kΩ, Resistor_SMD:R_0603_1608Metric, F.Cu at (111.6, 166.8)
- added R5: 10kΩ, Resistor_SMD:R_0603_1608Metric, F.Cu at (133.6, 120.8)
- added R5: 10kΩ, Resistor_SMD:R_0603_1608Metric, F.Cu at (89.6, 178.2)
- added R5: 10kΩ, Resistor_SMD:R_0603_1608Metric, F.Cu at (67.6, 97.8)
- added R5: 10kΩ, Resistor_SMD:R_0603_1608Metric, F.Cu at (89.6, 166.8)
- added R5: 10kΩ, Resistor_SMD:R_0603_1608Metric, F.Cu at (111.6, 143.8)
- added R5: 10kΩ, Resistor_SMD:R_0603_1608Metric, F.Cu at (89.6, 132.2)
- added R5: 10kΩ, Resistor_SMD:R_0603_1608Metric, F.Cu at (133.6, 97.8)
- added R5: 10kΩ, Resistor_SMD:R_0603_1608Metric, F.Cu at (67.6, 132.2)
- added R5: 10kΩ, Resistor_SMD:R_0603_1608Metric, F.Cu at (133.6, 143.8)
- added R5: 10kΩ, Resistor_SMD:R_0603_1608Metric, F.Cu at (67.6, 166.8)
- added R5: 10kΩ, Resistor_SMD:R_0603_1608Metric, F.Cu at (111.6, 109.2)
- added R5: 10kΩ, Resistor_SMD:R_0603_1608Metric, F.Cu at (133.6, 178.2)
- added R5: 10kΩ, Resistor_SMD:R_0603_1608Metric, F.Cu at (111.6, 132.2)
- added R5: 10kΩ, Resistor_SMD:R_0603_1608Metric, F.Cu at (111.6, 178.2)
- added R6: 100Ω, Resistor_SMD:R_0603_1608Metric, F.Cu at (74.4, 126.2)
- added R6: 100Ω, Resistor_SMD:R_0603_1608Metric, F.Cu at (74.4, 172.2)
- added R6: 100Ω, Resistor_SMD:R_0603_1608Metric, F.Cu at (74.4, 160.8)
- added R6: 100Ω, Resistor_SMD:R_0603_1608Metric, F.Cu at (118.4, 91.8)
- added R6: 100Ω, Resistor_SMD:R_0603_1608Metric, F.Cu at (140.4, 160.8)
- added R6: 100Ω, Resistor_SMD:R_0603_1608Metric, F.Cu at (118.4, 137.8)
- added R6: 100Ω, Resistor_SMD:R_0603_1608Metric, F.Cu at (140.4, 114.8)
- added R6: 100Ω, Resistor_SMD:R_0603_1608Metric, F.Cu at (140.4, 126.2)
- added R6: 100Ω, Resistor_SMD:R_0603_1608Metric, F.Cu at (118.4, 126.2)
- added R6: 100Ω, Resistor_SMD:R_0603_1608Metric, F.Cu at (96.4, 160.8)
- added R6: 100Ω, Resistor_SMD:R_0603_1608Metric, F.Cu at (74.4, 103.2)
- added R6: 100Ω, Resistor_SMD:R_0603_1608Metric, F.Cu at (140.4, 91.8)
- added R6: 100Ω, Resistor_SMD:R_0603_1608Metric, F.Cu at (96.4, 126.2)
- added R6: 100Ω, Resistor_SMD:R_0603_1608Metric, F.Cu at (96.4, 149.2)
- added R6: 100Ω, Resistor_SMD:R_0603_1608Metric, F.Cu at (118.4, 160.8)
- added R6: 100Ω, Resistor_SMD:R_0603_1608Metric, F.Cu at (74.4, 114.8)
- added R6: 100Ω, Resistor_SMD:R_0603_1608Metric, F.Cu at (118.4, 114.8)
- added R6: 100Ω, Resistor_SMD:R_0603_1608Metric, F.Cu at (140.4, 137.8)
- added R6: 100Ω, Resistor_SMD:R_0603_1608Metric, F.Cu at (96.4, 114.8)
- added R6: 100Ω, Resistor_SMD:R_0603_1608Metric, F.Cu at (74.4, 137.8)
- added R6: 100Ω, Resistor_SMD:R_0603_1608Metric, F.Cu at (140.4, 172.2)
- added R6: 100Ω, Resistor_SMD:R_0603_1608Metric, F.Cu at (96.4, 91.8)
- added R6: 100Ω, Resistor_SMD:R_0603_1608Metric, F.Cu at (96.4, 103.2)
- added R6: 100Ω, Resistor_SMD:R_0603_1608Metric, F.Cu at (140.4, 103.2)
- added R6: 100Ω, Resistor_SMD:R_0603_1608Metric, F.Cu at (118.4, 103.2)
- added R6: 100Ω, Resistor_SMD:R_0603_1608Metric, F.Cu at (118.4, 172.2)
- added R6: 100Ω, Resistor_SMD:R_0603_1608Metric, F.Cu at (74.4, 149.2)
- added R6: 100Ω, Resistor_SMD:R_0603_1608Metric, F.Cu at (96.4, 172.2)
- added R6: 100Ω, Resistor_SMD:R_0603_1608Metric, F.Cu at (74.4, 91.8)
- added R6: 100Ω, Resistor_SMD:R_0603_1608Metric, F.Cu at (118.4, 149.2)
- added R6: 100Ω, Resistor_SMD:R_0603_1608Metric, F.Cu at (96.4, 137.8)
- added R6: 100Ω, Resistor_SMD:R_0603_1608Metric, F.Cu at (140.4, 149.2)
- added R7: 100Ω, Resistor_SMD:R_0603_1608Metric, F.Cu at (74.4, 113.2)
- added R7: 100Ω, Resistor_SMD:R_0603_1608Metric, F.Cu at (140.4, 136.2)
- added R7: 100Ω, Resistor_SMD:R_0603_1608Metric, F.Cu at (96.4, 147.8)
- added R7: 100Ω, Resistor_SMD:R_0603_1608Metric, F.Cu at (74.4, 136.2)
- added R7: 100Ω, Resistor_SMD:R_0603_1608Metric, F.Cu at (140.4, 90.2)
- added R7: 100Ω, Resistor_SMD:R_0603_1608Metric, F.Cu at (74.4, 147.8)
- added R7: 100Ω, Resistor_SMD:R_0603_1608Metric, F.Cu at (140.4, 147.8)
- added R7: 100Ω, Resistor_SMD:R_0603_1608Metric, F.Cu at (140.4, 113.2)
- added R7: 100Ω, Resistor_SMD:R_0603_1608Metric, F.Cu at (96.4, 136.2)
- added R7: 100Ω, Resistor_SMD:R_0603_1608Metric, F.Cu at (96.4, 101.8)
- added R7: 100Ω, Resistor_SMD:R_0603_1608Metric, F.Cu at (96.4, 113.2)
- added R7: 100Ω, Resistor_SMD:R_0603_1608Metric, F.Cu at (140.4, 101.8)
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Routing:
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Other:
- board size 92 x 92 mm -> 88 x 92 mm
- board text added: "3.3V"
- board text added: "5V"
- board text added: "BOOT"
- board text added: "CH552-DAPLink v1.0.0 @netetra07"
- board text added: "GND"
- board text added: "RST"
- board text added: "SWCLK"
- board text added: "SWDIO"
- board text added: "←V-Cut"
- board text removed: "<- V-Cut"
- board text removed: "CH552-DAPLink @netetra07"
